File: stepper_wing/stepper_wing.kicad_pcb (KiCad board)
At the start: 2 copper layers, 47 x 49.5 mm, 40 parts, among them U1 MCP44X1, U2 MCP23017, U3 DRV8825, U4 DRV8825, U5 DRV8825, U6 DRV8825

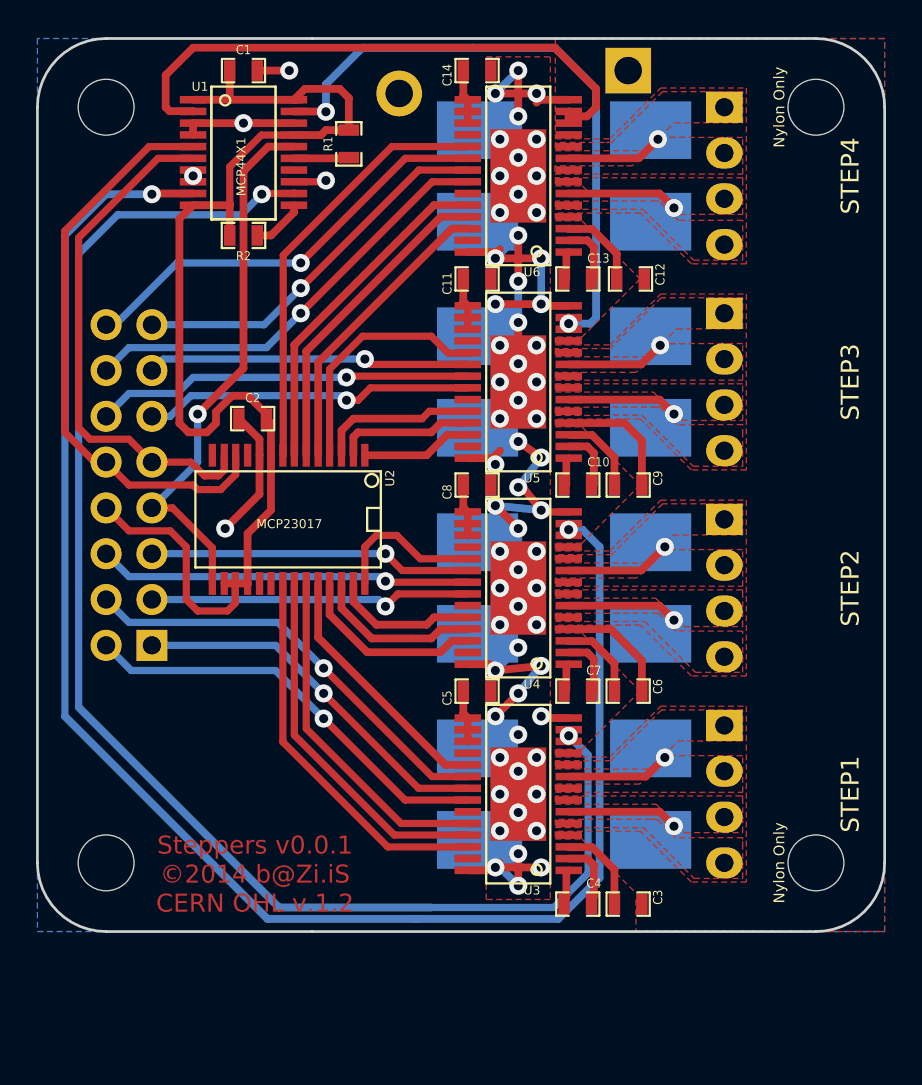
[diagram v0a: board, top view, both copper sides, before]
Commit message: try alt layout
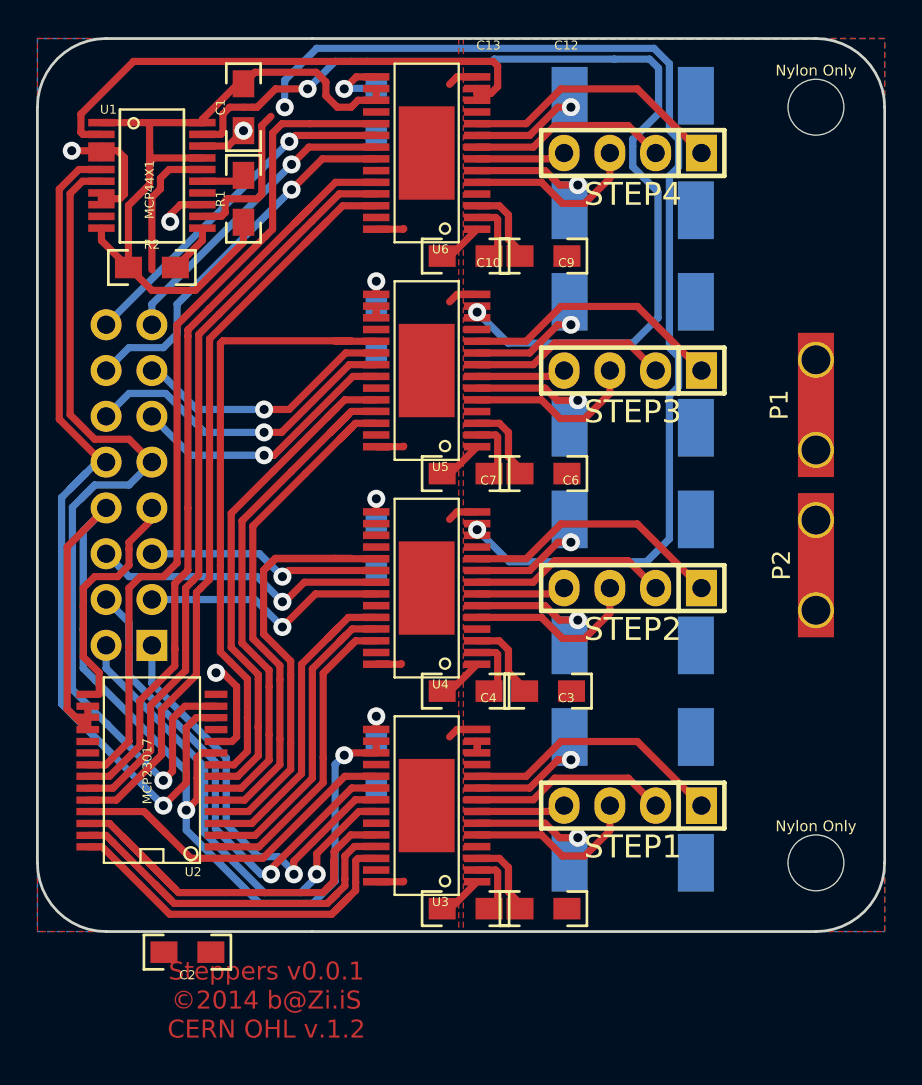
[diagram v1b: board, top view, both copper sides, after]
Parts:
- removed the Nylon Only at (106.4, 80.5)
- removed the Nylon Only at (106.4, 122.4)
- removed WINGPWR1: WINGPWR, Connect:bornier2
- added P1: CONN_1, Local:TabRA, F.Cu at (145.8, 97.0)
- added P2: CONN_1, Local:TabRA, F.Cu at (145.8, 105.9)
- C1, C10, C12, C13, C2, C3, C4, C6, C7, C9: footprint SMD_Packages:SMD-0603_c -> Local:0805C
- C11, C14, C5, C8: footprint SMD_Packages:SMD-0603_c -> Local:0805C; moved to B.Cu
- R1, R2: footprint SMD_Packages:SMD-0603_r -> Local:0805R
- R10, R3, R4, R5, R6, R7, R8, R9: footprint Resistors_SMD:Resistor_SMD2512_HandSoldering -> Resistors_SMD:R_2512
- STEP1, STEP2, STEP3, STEP4: footprint Pin_Headers:Pin_Header_Angled_1x04 -> Pin_Headers:Pin_Header_Straight_1x04
- moved C2 29.8 mm to (110.9, 127.4), turned to 0 degrees
- moved U2 15.9 mm to (109.0, 117.3), turned to 90 degrees
- moved C5 6.91 mm to (121.4, 117.0), turned to 270 degrees
- moved R1 6.59 mm to (114.0, 85.6), turned to 90 degrees
- moved C8 6.56 mm to (121.4, 104.9), turned to 270 degrees
- moved C13 6.35 mm to (126.4, 88.8)
- moved C10 6.26 mm to (126.4, 100.8)
- moved C11 6.25 mm to (121.4, 92.8), turned to 270 degrees
- moved C4 6.23 mm to (126.4, 125.0)
- moved C7 6.22 mm to (126.4, 112.9)
- moved C14 6.04 mm to (121.4, 80.8), turned to 270 degrees
- moved R2 5.38 mm to (109.0, 89.4)
- moved STEP4 5.24 mm to (135.6, 83.1), turned to 180 degrees
- moved U1 5.24 mm to (109.0, 84.3)
- moved U6 5.24 mm to (124.2, 83.1)
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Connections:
- U2 pad 1: /Stepper2/MODE2 -> /Stepper1/MODE2
- U2 pad 2: /Stepper2/MODE1 -> /Stepper1/MODE1
- U2 pad 21: /Stepper0/MODE2 -> /Stepper3/DECAY
- U2 pad 22: /Stepper0/MODE1 -> /Stepper3/MODE0
- U2 pad 23: /Stepper0/MODE0 -> /Stepper3/MODE1
- U2 pad 24: /Stepper0/DECAY -> /Stepper3/MODE2
- U2 pad 25: /Stepper1/MODE2 -> /Stepper0/DECAY
- U2 pad 26: /Stepper1/MODE1 -> /Stepper0/MODE0
- U2 pad 27: /Stepper1/MODE0 -> /Stepper0/MODE1
- U2 pad 28: /Stepper1/DECAY -> /Stepper0/MODE2
- U2 pad 3: /Stepper2/MODE0 -> /Stepper1/MODE0
- U2 pad 4: /Stepper2/DECAY -> /Stepper1/DECAY
- U2 pad 5: /Stepper3/MODE2 -> /Stepper2/MODE2
- U2 pad 6: /Stepper3/MODE1 -> /Stepper2/MODE1
- U2 pad 7: /Stepper3/MODE0 -> /Stepper2/MODE0
- U2 pad 8: /Stepper3/DECAY -> /Stepper2/DECAY
- U3 pad 16: Net-(C5-Pad1) -> +3.3V
- U3 pad 17: Net-(C5-Pad1) -> +3.3V
- U3 pad 5: Net-(STEP1-Pad4) -> Net-(STEP1-Pad3)
- U3 pad 7: Net-(STEP1-Pad3) -> Net-(STEP1-Pad4)
- U4 pad 16: Net-(C8-Pad1) -> +3.3V
- U4 pad 17: Net-(C8-Pad1) -> +3.3V
- U4 pad 5: Net-(STEP2-Pad4) -> Net-(STEP2-Pad3)
- U4 pad 7: Net-(STEP2-Pad3) -> Net-(STEP2-Pad4)
- U5 pad 16: Net-(C11-Pad1) -> +3.3V
- U5 pad 17: Net-(C11-Pad1) -> +3.3V
- U5 pad 5: Net-(STEP3-Pad4) -> Net-(STEP3-Pad3)
- U5 pad 7: Net-(STEP3-Pad3) -> Net-(STEP3-Pad4)
- U6 pad 16: Net-(C14-Pad1) -> +3.3V
- U6 pad 17: Net-(C14-Pad1) -> +3.3V
- U6 pad 5: Net-(STEP4-Pad4) -> Net-(STEP4-Pad3)
- U6 pad 7: Net-(STEP4-Pad3) -> Net-(STEP4-Pad4)
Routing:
- net GND: track 105.9 -> 32.6 mm, vias 66 -> 4
- net /Stepper0/PW: track 80.9 -> 9.35 mm, vias 2 -> 0
- net +3.3V: track 69.4 -> 103.7 mm, vias 0 -> 2
- net /Stepper1/PW: track 91.3 -> 63.7 mm
- net /Stepper3/MODE2: track 16.5 -> 43.3 mm
- net /Stepper3/MODE0: track 19.0 -> 42.9 mm
- net /Stepper3/MODE1: track 17.8 -> 41.6 mm
- net /Stepper3/DECAY: track 23.8 -> 46.6 mm
- net /Stepper2/MODE2: track 6.18 -> 28.5 mm
- net /Stepper2/DECAY: track 13.6 -> 35.0 mm
- net /Stepper2/MODE1: track 7.69 -> 28.9 mm
- net /SDA: track 28.8 -> 50.0 mm, vias 0 -> 1
- net /SCL: track 32.4 -> 53.5 mm, vias 0 -> 1
- net /Stepper1/DECAY: track 8.54 -> 28.2 mm
- net /Stepper2/MODE0: track 8.82 -> 28.5 mm
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- removed copper zone on F.Cu, net Net-(STEP1-Pad1)
- removed copper zone on F.Cu, net Net-(STEP1-Pad2)
- removed copper zone on F.Cu, net Net-(STEP1-Pad3)
- removed copper zone on F.Cu, net Net-(STEP1-Pad4)
- removed copper zone on F.Cu, net Net-(STEP2-Pad1)
- removed copper zone on F.Cu, net Net-(STEP2-Pad2)
- removed copper zone on F.Cu, net Net-(STEP2-Pad3)
- removed copper zone on F.Cu, net Net-(STEP2-Pad4)
- removed copper zone on F.Cu, net Net-(STEP3-Pad1)
- removed copper zone on F.Cu, net Net-(STEP3-Pad2)
- removed copper zone on F.Cu, net Net-(STEP3-Pad3)
- removed copper zone on F.Cu, net Net-(STEP3-Pad4)
- removed copper zone on F.Cu, net Net-(STEP4-Pad1)
- removed copper zone on F.Cu, net Net-(STEP4-Pad2)
- removed copper zone on F.Cu, net Net-(STEP4-Pad3)
- removed copper zone on F.Cu, net Net-(STEP4-Pad4)
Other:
- net class Default: trace_width 0.4318 -> 0.4
